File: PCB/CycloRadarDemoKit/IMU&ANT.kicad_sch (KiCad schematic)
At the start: 20 parts, among them J101 ANT_JTAG, U302 D52MxxM8, U501 MPU-6050, U502 LSM6DSM

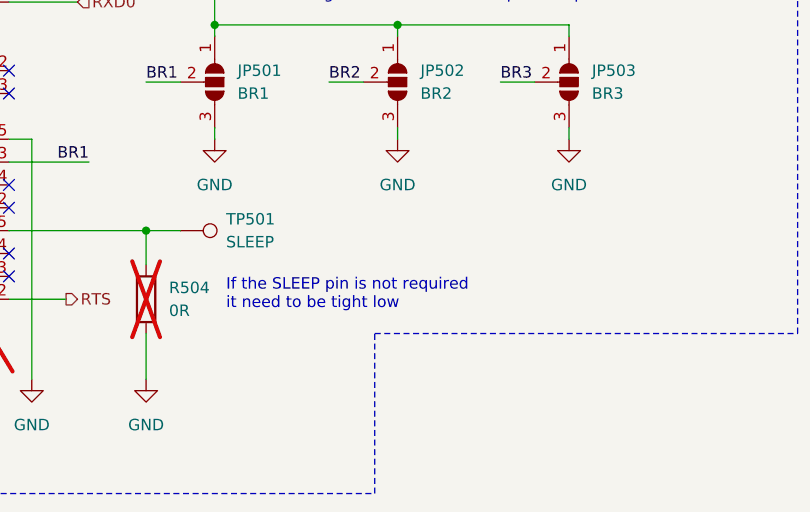
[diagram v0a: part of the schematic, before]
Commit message: PCB ready for review
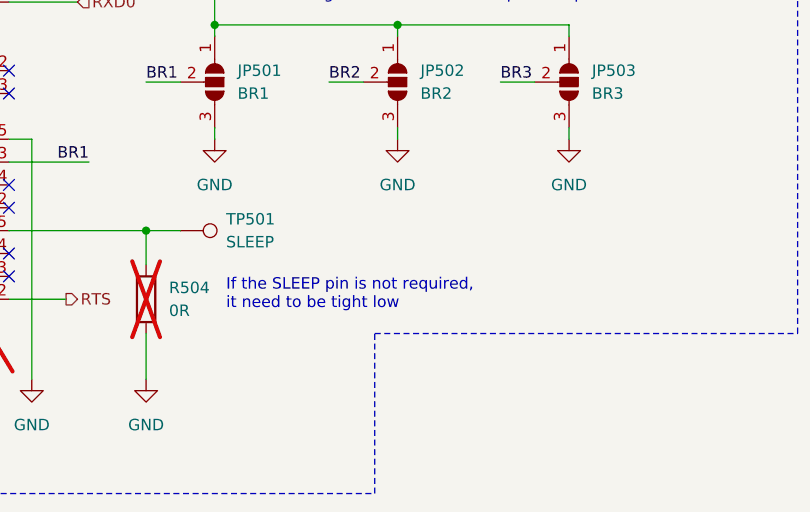
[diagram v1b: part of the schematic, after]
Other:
- note added: "If the SLEEP pin is not required, it need to be tight low"
- note removed: "If the SLEEP pin is not required it need to be tight low"
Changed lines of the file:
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@@
     (effects (font (size 2 2) (thickness 0.4) bold) (justify left bottom))
   )
-  (text "If the SLEEP pin is not required \nit need to be tight low"
+  (text "If the SLEEP pin is not required,\nit need to be tight low"
     (at 148.59 158.75 0)
     (effects (font (size 1.27 1.27)) (justify left bottom))

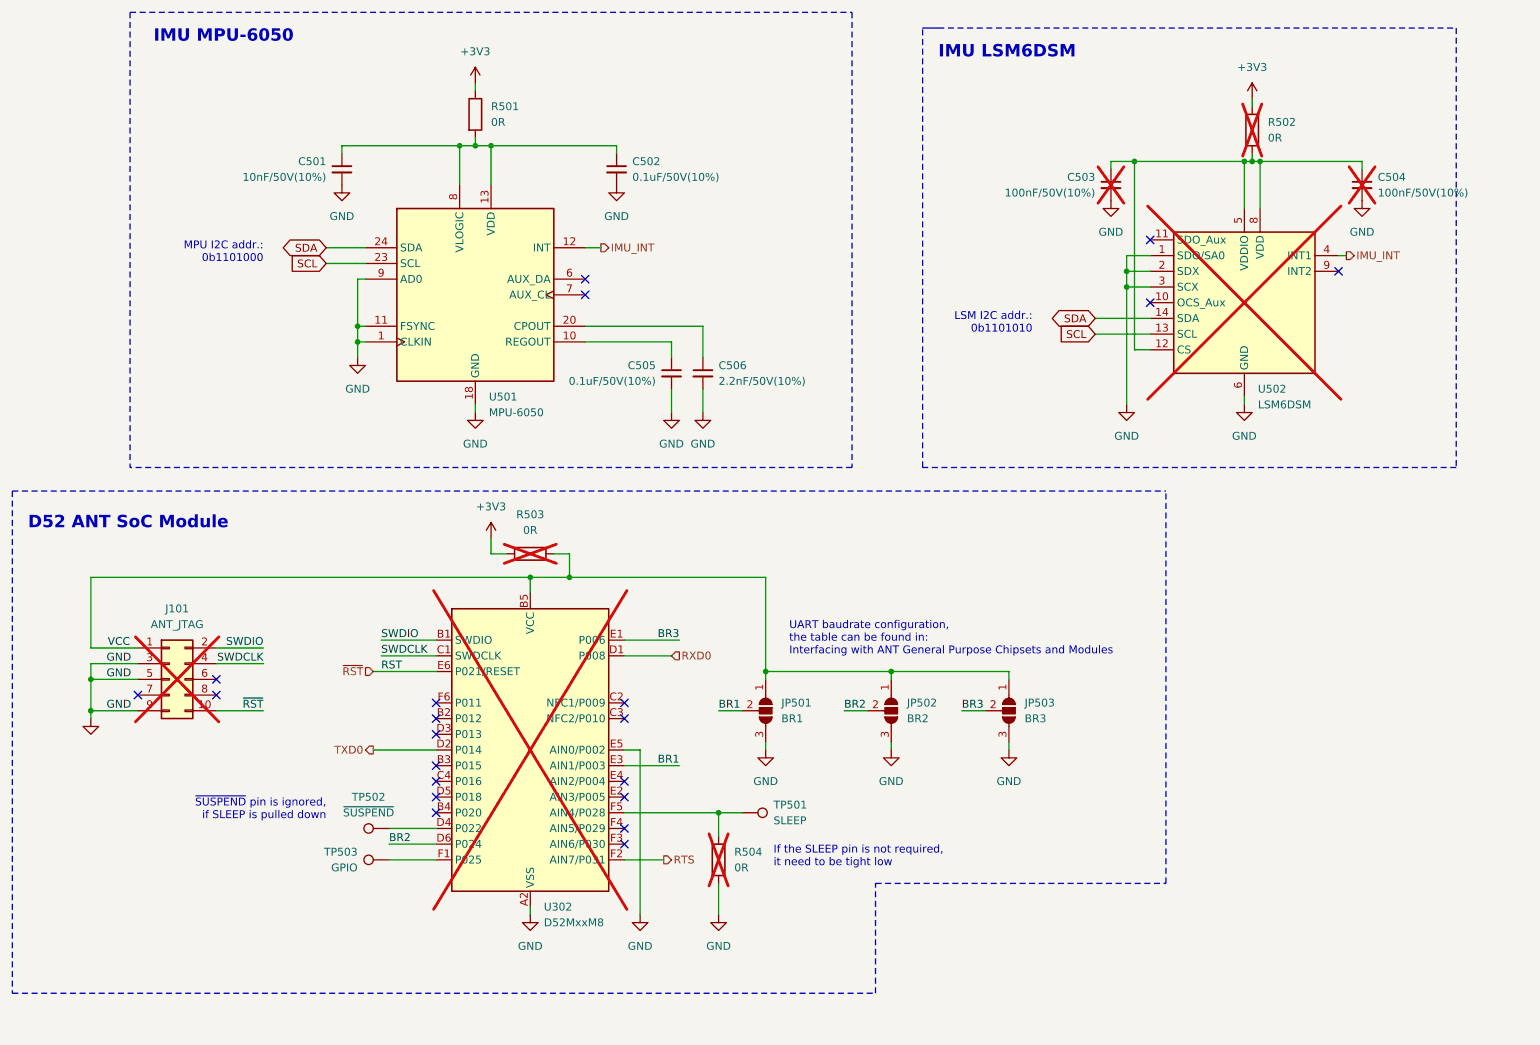
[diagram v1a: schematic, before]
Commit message: PCB after review
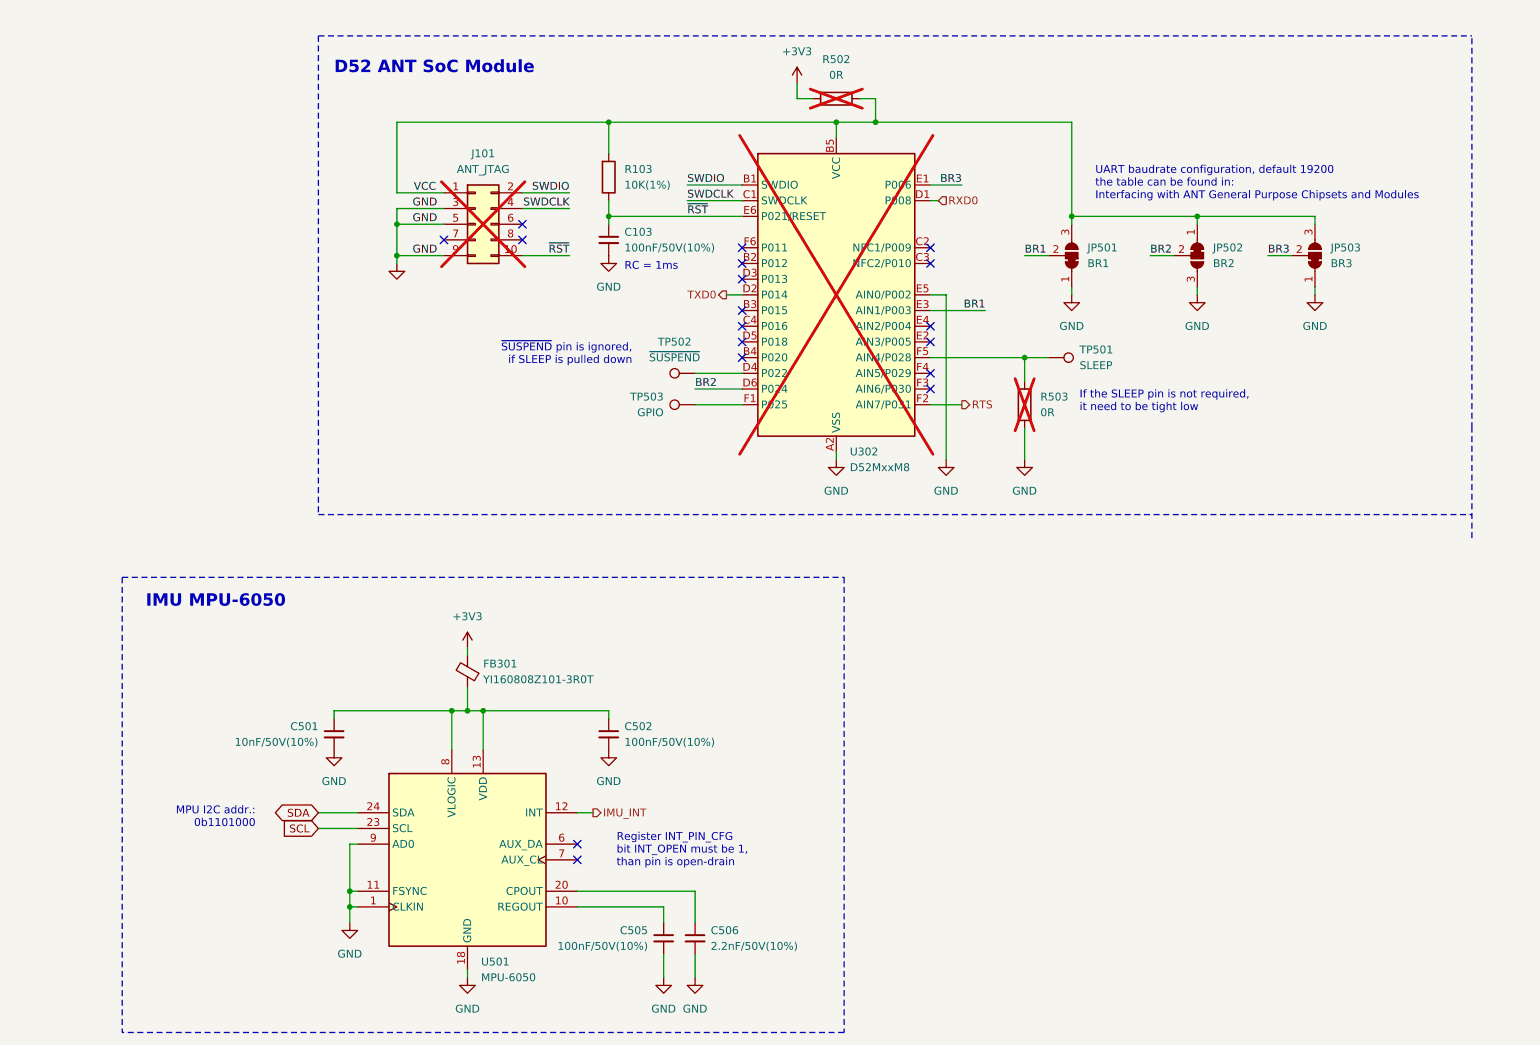
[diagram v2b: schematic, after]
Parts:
- removed C503, C504: 100nF/50V(10%), Capacitor_SMD:C_0805_2012Metric, symbol Device:C_Small
- removed JP502: BR2, Jumper:SolderJumper-3_P1.3mm_Open_RoundedPad1.0x1.5mm_NumberLabels, symbol Jumper:SolderJumper_3_Open
- removed JP503: BR3, Jumper:SolderJumper-3_P1.3mm_Open_RoundedPad1.0x1.5mm_NumberLabels, symbol Jumper:SolderJumper_3_Open
- removed R501, R502: 0R, Resistor_SMD:R_0805_2012Metric, symbol Device:R
- removed U502: LSM6DSM, Package_LGA:LGA-14_3x2.5mm_P0.5mm_LayoutBorder3x4y, symbol Sensor_Motion:LSM6DSM
- added C103: 100nF/50V(10%), Capacitor_SMD:C_0603_1608Metric, symbol Device:C_Small
- added FB301: YI160808Z101-3R0T, Resistor_SMD:R_0603_1608Metric, symbol Device:FerriteBead_Small
- added JP502: BR2, Jumper:SolderJumper-3_P1.3mm_Bridged12_RoundedPad1.0x1.5mm_NumberLabels, symbol Jumper:SolderJumper_3_Bridged12
- added JP503: BR3, Jumper:SolderJumper-3_P1.3mm_Bridged12_RoundedPad1.0x1.5mm_NumberLabels, symbol Jumper:SolderJumper_3_Bridged12
- added R103: 10K(1%), Resistor_SMD:R_0603_1608Metric, symbol Device:R
- C501: footprint Capacitor_SMD:C_0603_1608Metric -> Capacitor_SMD:C_0402_1005Metric; LCSC C57112 -> C15195
- C502, C505: value 0.1uF/50V(10%) -> 100nF/50V(10%)
- JP501: footprint Jumper:SolderJumper-3_P1.3mm_Open_RoundedPad1.0x1.5mm_NumberLabels -> Jumper:SolderJumper-3_P1.3mm_Bridged12_RoundedPad1.0x1.5mm_NumberLabels; symbol Jumper:SolderJumper_3_Open -> Jumper:SolderJumper_3_Bridged12
- TP501, TP502, TP503: footprint (none) -> TestPoint:TestPoint_Pad_D2.0mm
- renumbered R503 to R502, R504 to R503
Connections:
- net +3V3: now also FB301.2
- net BR2: now also JP502.2 (C)
- net BR3: now also JP503.2 (C)
- net GND: now also JP501.1 (A), C103.2, JP502.3 (B), JP503.1 (A); no longer JP501.3 (B)
- net VCC: now also JP501.3 (B), JP502.1 (A), JP503.3 (B), R103.2; no longer JP501.1 (A)
- net ~{RST}: now also C103.1, R103.1
- net at C501.1, C502.1, U501.13 (VDD)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: now also FB301.1
- no-connect marks 21 -> 18
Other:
- note added: "RC = 1ms"
- note added: "Register INT_PIN_CFG bit INT_OPEN must be 1, than pin is open-drain"
- note added: "UART baudrate configuration, default 19200 the table can be found in: Interfacing with ANT General Purpose Chipsets and Modules"
- note removed: "IMU LSM6DSM"
- note removed: "LSM I2C addr.: 0b1101010"
- note removed: "UART baudrate configuration, the table can be found in: Interfacing with ANT General Purpose Chipsets and Modules"
- company: (none) -> ALPS Electric Czech, s.r.o.
- title: (none) -> Safety Ride Radar Sensor
- moved on the sheet: C501, C502, C505, C506, J101, R502, R503, TP501, TP502, TP503, U302, U501
